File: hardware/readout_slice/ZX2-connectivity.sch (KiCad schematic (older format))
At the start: 13 parts

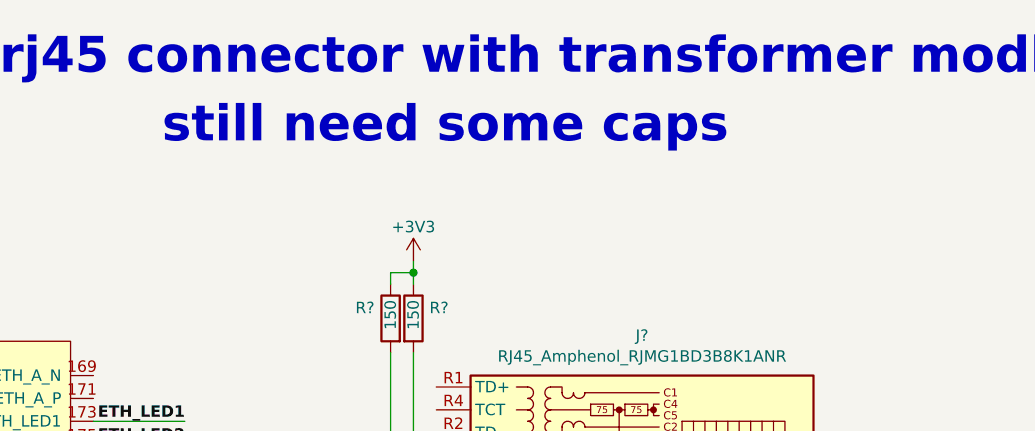
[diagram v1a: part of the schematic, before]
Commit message: more progress on readout_slice
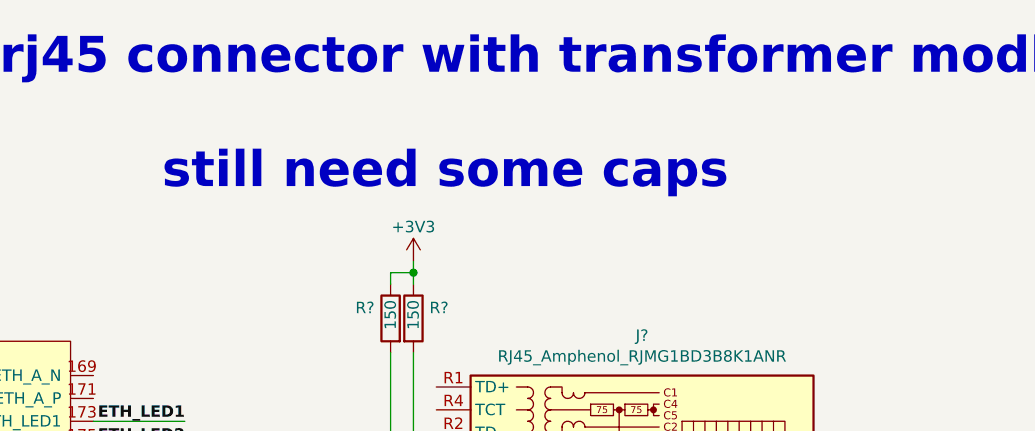
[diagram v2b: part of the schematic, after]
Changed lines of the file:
@@
 Text Notes 4850 150  0    157  ~ 31
 magjack for eth rj45 connector with transformer modled into it\n
-Text Notes 7550 450  0    157  ~ 31
+Text Notes 7550 650  0    157  ~ 31
 still need some caps\n
 $Comp

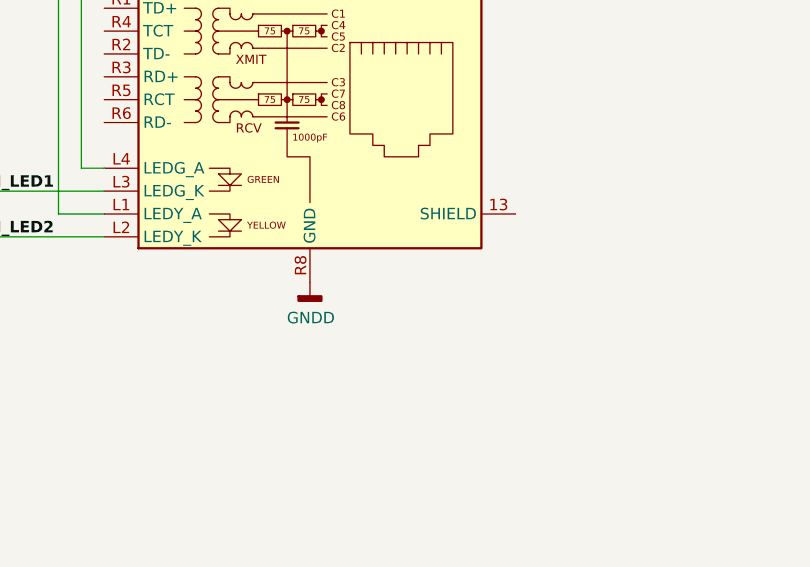
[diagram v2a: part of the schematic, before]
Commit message: auto push run at Fri Apr  9 14:02:10 EDT 2021
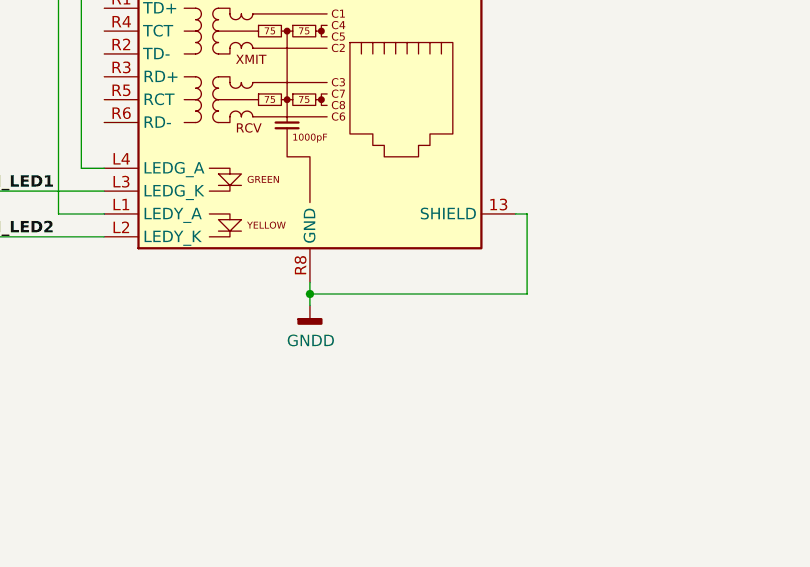
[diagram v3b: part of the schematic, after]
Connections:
- net GNDD: now also J?.13 (SHIELD)
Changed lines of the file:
@@
 $Descr A4 11693 8268
 encoding utf-8
-Sheet 5 16
+Sheet 4 15
 Title ""
 Date ""
@@
 L power:GNDD #PWR?
 U 1 1 60EE4CD2
-P 9650 2700
+P 9650 2800
 AR Path="/60EE4CD2" Ref="#PWR?"  Part="1"
 AR Path="/608B2FC0/60EE4CD2" Ref="#PWR?"  Part="1"
 AR Path="/60AD0200/60B2D848/60EE4CD2" Ref="#PWR?"  Part="1"
 AR Path="/607155C8/60EE4CD2" Ref="#PWR?"  Part="1"
-F 0 "#PWR?" H 9650 2450 50  0001 C CNN
-F 1 "GNDD" H 9654 2545 50  0000 C CNN
-F 2 "" H 9650 2700 50  0001 C CNN
-F 3 "" H 9650 2700 50  0001 C CNN
-	1    9650 2700
+F 0 "#PWR?" H 9650 2550 50  0001 C CNN
+F 1 "GNDD" H 9654 2645 50  0000 C CNN
+F 2 "" H 9650 2800 50  0001 C CNN
+F 3 "" H 9650 2800 50  0001 C CNN
+	1    9650 2800
 	1    0    0    -1
 $EndComp
@@
 Wire Wire Line
 	8150 2300 8750 2300
+Wire Wire Line
+	9650 2800 9650 2750
+Wire Wire Line
+	9650 2750 10600 2750
+Wire Wire Line
+	10600 2750 10600 2400
+Wire Wire Line
+	10600 2400 10550 2400
+Connection ~ 9650 2750
+Wire Wire Line
+	9650 2750 9650 2700
 $EndSCHEMATC

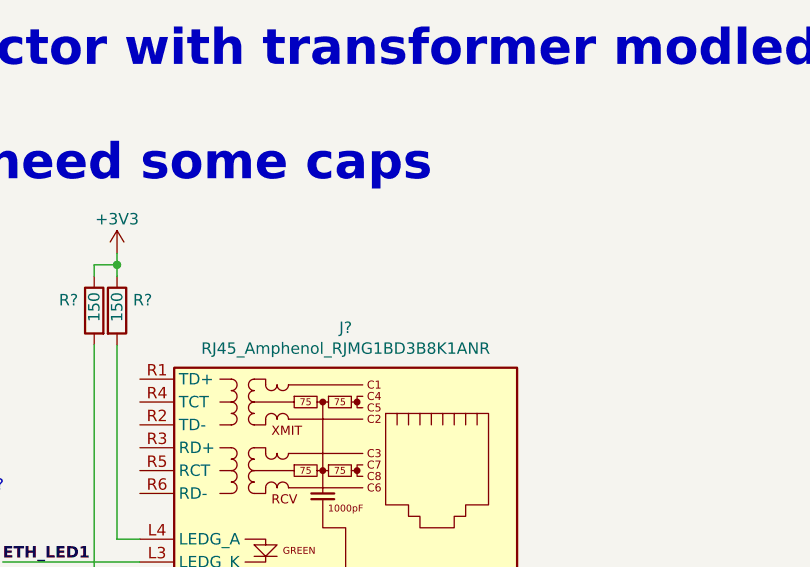
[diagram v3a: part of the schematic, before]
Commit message: auto push run at Fri Apr  9 16:59:37 EDT 2021
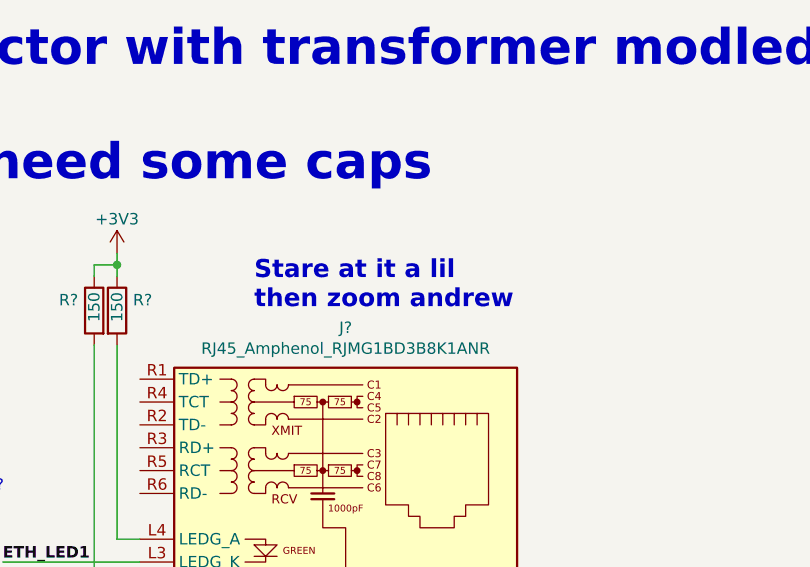
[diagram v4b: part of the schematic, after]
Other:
- note added: "Stare at it a lil\nthen zoom andrew"
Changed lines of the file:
@@
 $Descr A4 11693 8268
 encoding utf-8
-Sheet 4 15
+Sheet 3 15
 Title ""
 Date ""
@@
 Wire Wire Line
 	9650 2750 9650 2700
+Text Notes 9250 1200 0    79   ~ 16
+Stare at it a lil\nthen zoom andrew
 $EndSCHEMATC
